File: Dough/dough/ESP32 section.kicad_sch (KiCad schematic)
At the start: 27 parts, among them J12 Conn_01x10_Pin, J401 SD CARD, Q1 2N7002, Q4 2N7002, SW2 ESP32 BOOT, SW4 ESP32 RST, U9 ESP32-S3-WROOM-1

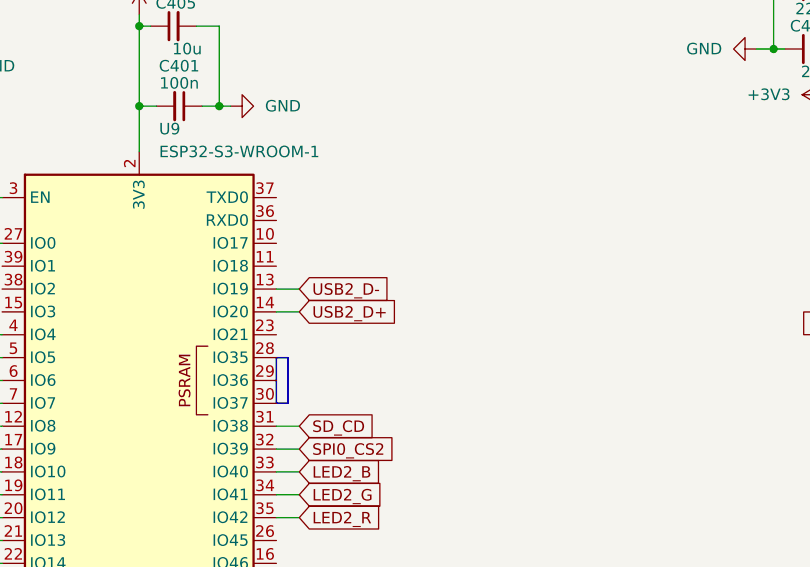
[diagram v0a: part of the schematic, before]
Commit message: started routing
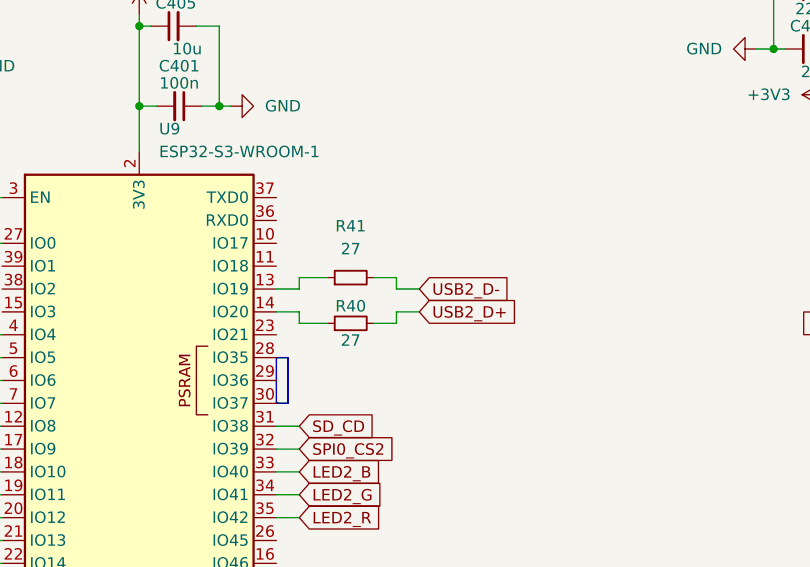
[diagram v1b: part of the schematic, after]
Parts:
- added R40, R41: 27, Resistor_SMD:R_0603_1608Metric_Pad0.98x0.95mm_HandSolder, symbol Device:R_Small
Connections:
- net USB2_D+: now also R40.2; no longer U9.14 (IO20)
- net USB2_D-: now also R41.2; no longer U9.13 (IO19)
- new net: R41.1, U9.13 (IO19)
- new net: R40.1, U9.14 (IO20)
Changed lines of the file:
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@@
+	(wire
+		(pts
+			(xy 154.94 79.375) (xy 151.765 79.375)
+		)
+		(stroke
+			(width 0)
+			(type default)
+		)
+	)
 	(wire
 		(pts
@@
 	(wire
 		(pts
+			(xy 162.56 74.295) (xy 162.56 75.565)
+		)
+		(stroke
+			(width 0)
+			(type default)
+		)
+	)
+	(wire
+		(pts
 			(xy 102.235 66.04) (xy 102.235 73.025)
 		)
@@
 	(wire
 		(pts
+			(xy 149.225 75.565) (xy 151.765 75.565)
+		)
+		(stroke
+			(width 0)
+			(type default)
+		)
+	)
+	(wire
+		(pts
 			(xy 92.075 63.5) (xy 92.075 50.8)
 		)
@@
 	(wire
 		(pts
+			(xy 160.02 79.375) (xy 162.56 79.375)
+		)
+		(stroke
+			(width 0)
+			(type default)
+		)
+	)
+	(wire
+		(pts
 			(xy 204.47 48.895) (xy 205.74 48.895)
 		)
@@
 	(wire
 		(pts
+			(xy 151.765 75.565) (xy 151.765 74.295)
+		)
+		(stroke
+			(width 0)
+			(type default)
+		)
+	)
+	(wire
+		(pts
 			(xy 219.075 84.455) (xy 219.075 81.915)
 		)
@@
 	(wire
 		(pts
+			(xy 151.765 74.295) (xy 154.94 74.295)
+		)
+		(stroke
+			(width 0)
+			(type default)
+		)
+	)
+	(wire
+		(pts
 			(xy 116.84 80.645) (xy 118.745 80.645)
 		)
@@
 	(wire
 		(pts
+			(xy 151.765 78.105) (xy 149.225 78.105)
+		)
+		(stroke
+			(width 0)
+			(type default)
+		)
+	)
+	(wire
+		(pts
 			(xy 204.47 29.845) (xy 204.47 34.925)
 		)
@@
 	(wire
 		(pts
+			(xy 162.56 75.565) (xy 165.1 75.565)
+		)
+		(stroke
+			(width 0)
+			(type default)
+		)
+	)
+	(wire
+		(pts
 			(xy 45.085 21.59) (xy 49.53 21.59)
 		)
@@
 	(wire
 		(pts
+			(xy 151.765 79.375) (xy 151.765 78.105)
+		)
+		(stroke
+			(width 0)
+			(type default)
+		)
+	)
+	(wire
+		(pts
 			(xy 151.765 98.425) (xy 149.225 98.425)
 		)
@@
 	(wire
 		(pts
-			(xy 151.765 78.105) (xy 149.225 78.105)
+			(xy 160.02 74.295) (xy 162.56 74.295)
 		)
 		(stroke
@@
 	(wire
 		(pts
+			(xy 162.56 78.105) (xy 165.1 78.105)
+		)
+		(stroke
+			(width 0)
+			(type default)
+		)
+	)
+	(wire
+		(pts
 			(xy 70.485 55.88) (xy 76.2 55.88)
 		)
@@
 	(wire
 		(pts
-			(xy 151.765 75.565) (xy 149.225 75.565)
+			(xy 162.56 79.375) (xy 162.56 78.105)
 		)
 		(stroke
@@
 	(global_label "USB2_D+"
 		(shape input)
-		(at 151.765 78.105 0)
+		(at 165.1 78.105 0)
 		(fields_autoplaced yes)
 		(effects
@@
 		)
 		(property "Intersheetrefs" "${INTERSHEET_REFS}"
-			(at 163.5797 78.105 0)
+			(at 176.9147 78.105 0)
 			(effects
 				(font
@@
 	(global_label "USB2_D-"
 		(shape input)
-		(at 151.765 75.565 0)
+		(at 165.1 75.565 0)
 		(fields_autoplaced yes)
 		(effects
@@
 		)
 		(property "Intersheetrefs" "${INTERSHEET_REFS}"
-			(at 163.5797 75.565 0)
+			(at 176.9147 75.565 0)
 			(effects
 				(font
@@
 	)
 	(symbol
+		(lib_id "Device:R_Small")
+		(at 157.48 74.295 90)
+		(unit 1)
+		(exclude_from_sim no)
+		(in_bom yes)
+		(on_board yes)
+		(dnp no)
+		(fields_autoplaced yes)
+		(property "Reference" "R41"
+			(at 157.48 68.58 90)
+			(effects
+				(font
+					(size 1.27 1.27)
+				)
+			)
+		)
+		(property "Value" "27"
+			(at 157.48 71.12 90)
+			(effects
+				(font
+					(size 1.27 1.27)
+				)
+			)
+		)
+		(property "Footprint" "Resistor_SMD:R_0603_1608Metric_Pad0.98x0.95mm_HandSolder"
+			(at 157.48 74.295 0)
+			(effects
+				(font
+					(size 1.27 1.27)
+				)
+				(hide yes)
+			)
+		)
+		(property "Datasheet" "~"
+			(at 157.48 74.295 0)
+			(effects
+				(font
+					(size 1.27 1.27)
+				)
+				(hide yes)
+			)
+		)
+		(property "Description" "Resistor, small symbol"
+			(at 157.48 74.295 0)
+			(effects
+				(font
+					(size 1.27 1.27)
+				)
+				(hide yes)
+			)
+		)
+		(pin "2"
+		)
+		(pin "1"
+		)
+		(instances
+			(project "dough"
+				(path "/4fefffc5-b577-4f4a-9ede-53ada2aa57cf/22e4c3eb-dc28-4f86-950b-d0bb031ef536"
+					(reference "R41")
+					(unit 1)
+				)
+			)
+		)
+	)
+	(symbol
 		(lib_id "power:GND")
 		(at 81.28 73.025 270)
@@
 					(unit 1)
 				)
+			)
+		)
+	)
+	(symbol
+		(lib_id "Device:R_Small")
+		(at 157.48 79.375 90)
+		(unit 1)
+		(exclude_from_sim no)
+		(in_bom yes)
+		(on_board yes)
+		(dnp no)
+		(property "Reference" "R40"
+			(at 157.48 77.47 90)
+			(effects
+				(font
+					(size 1.27 1.27)
+				)
+			)
+		)
+		(property "Value" "27"
+			(at 157.48 81.28 90)
+			(effects
+				(font
+					(size 1.27 1.27)
+				)
+			)
+		)
+		(property "Footprint" "Resistor_SMD:R_0603_1608Metric_Pad0.98x0.95mm_HandSolder"
+			(at 157.48 79.375 0)
+			(effects
+				(font
+					(size 1.27 1.27)
+				)
+				(hide yes)
+			)
+		)
+		(property "Datasheet" "~"
+			(at 157.48 79.375 0)
+			(effects
+				(font
+					(size 1.27 1.27)
+				)
+				(hide yes)
+			)
+		)
+		(property "Description" "Resistor, small symbol"
+			(at 157.48 79.375 0)
+			(effects
+				(font
+					(size 1.27 1.27)
+				)
+				(hide yes)
+			)
+		)
+		(pin "2"
+		)
+		(pin "1"
+		)
+		(instances
+			(project "dough"
+				(path "/4fefffc5-b577-4f4a-9ede-53ada2aa57cf/22e4c3eb-dc28-4f86-950b-d0bb031ef536"
+					(reference "R40")
+					(unit 1)
+				)

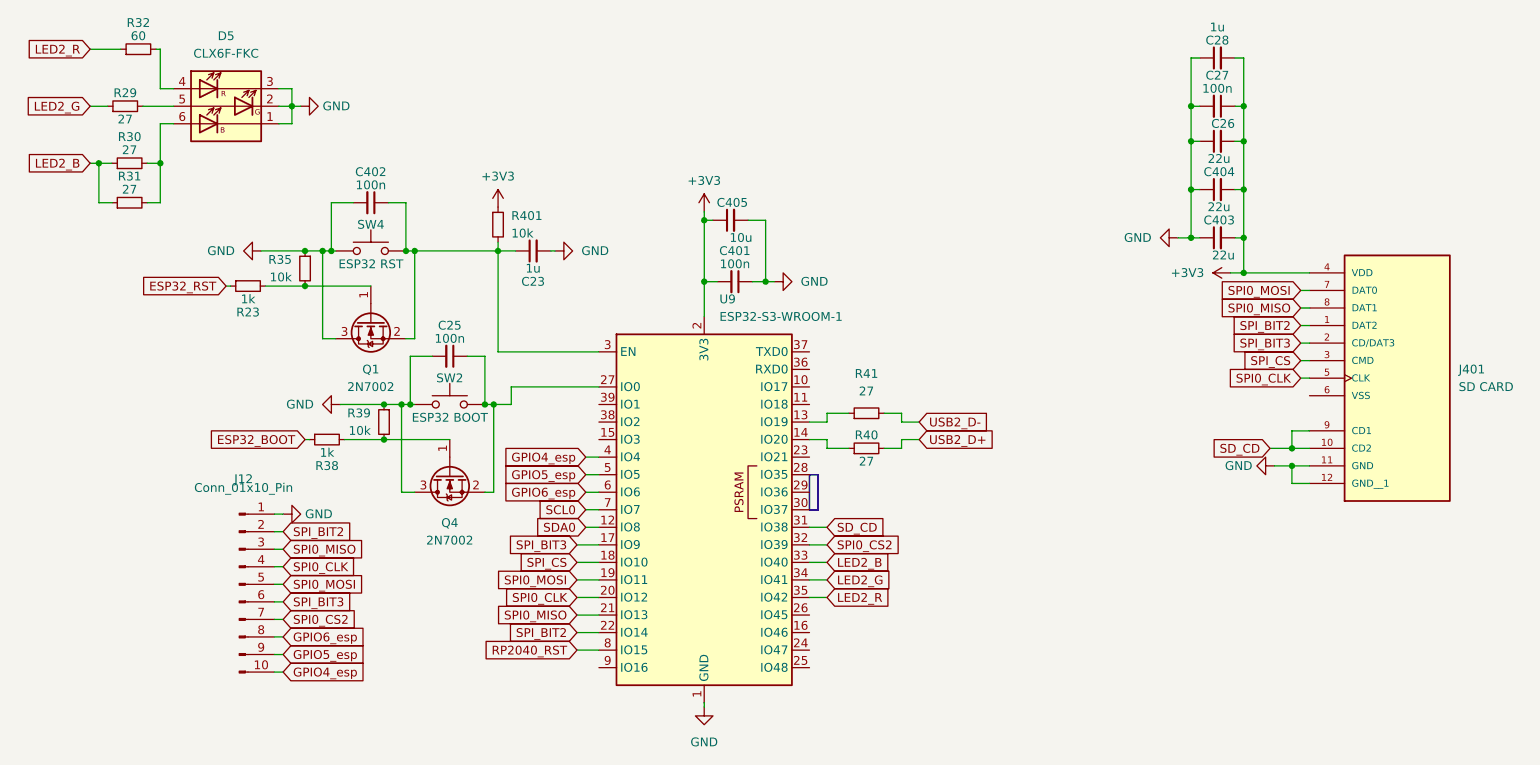
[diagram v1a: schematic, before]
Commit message: pre prod 1
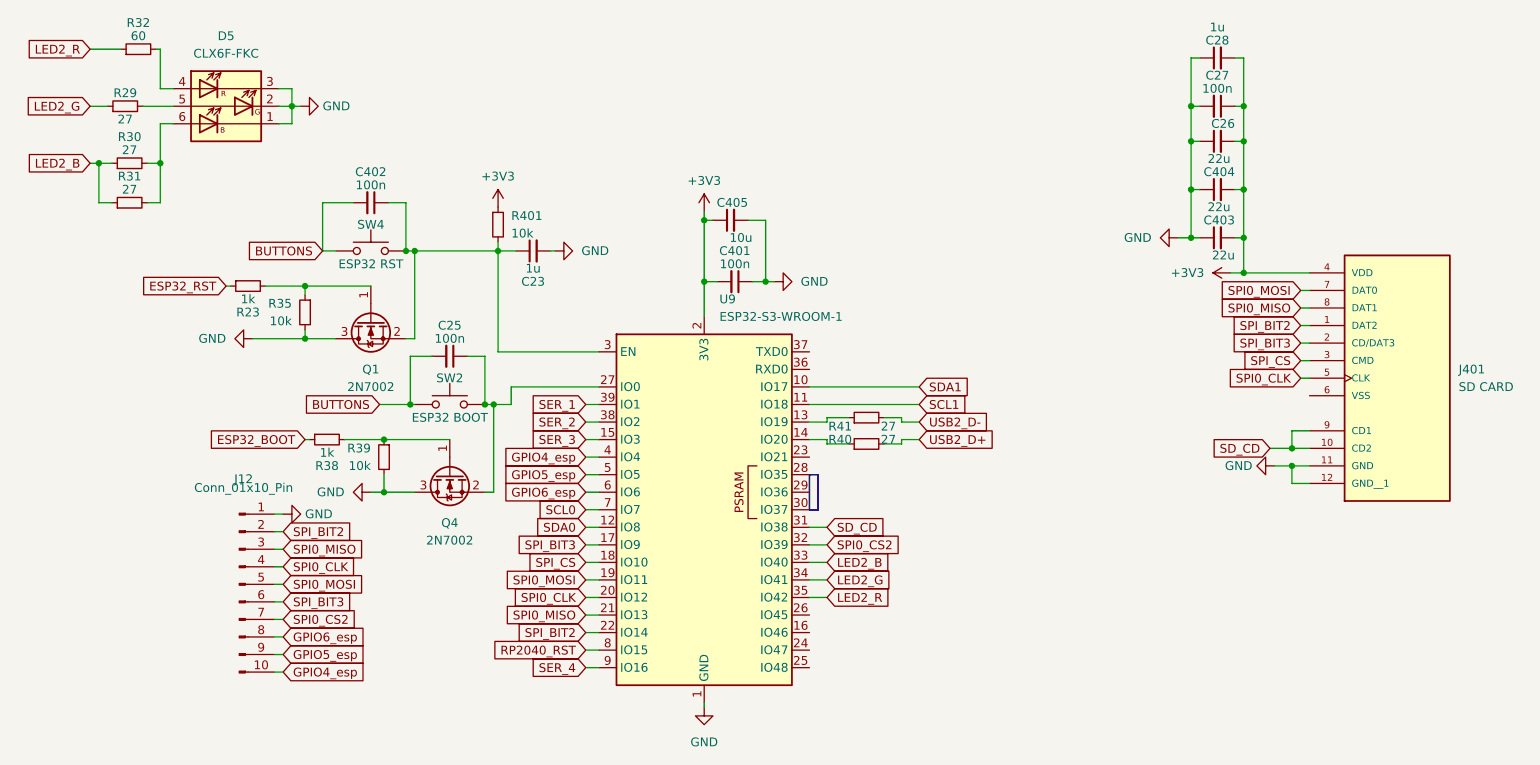
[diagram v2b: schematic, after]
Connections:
- net GND: now also R35.2, R39.2; no longer C25.2, C402.2, R35.1, R39.1, SW2.1, SW4.1
- net at Q1.1 (G), R23.2: now also R35.1; no longer R35.2
- net at Q4.1 (G), R38.2: now also R39.1; no longer R39.2
- net SDA1: now reaches U9.10 (IO17)
- net SCL1: now reaches U9.11 (IO18)
- net SER_3: now reaches U9.15 (IO3)
- net SER_2: now reaches U9.38 (IO2)
- net SER_1: now reaches U9.39 (IO1)
- net SER_4: now reaches U9.9 (IO16)
- new net BUTTONS: C25.2, C402.2, SW2.1, SW4.1
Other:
- moved on the sheet: R40, R41

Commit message: dough First production run
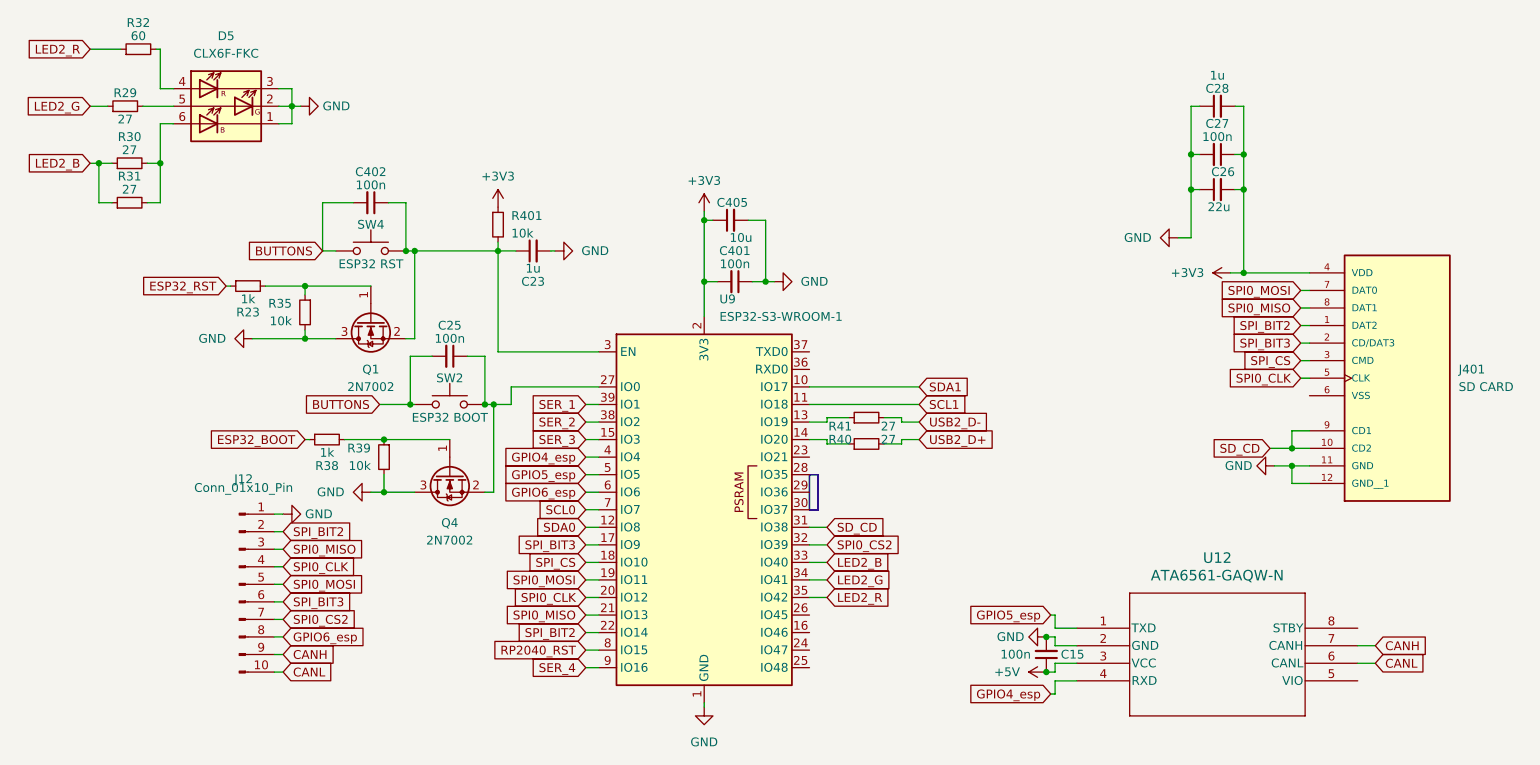
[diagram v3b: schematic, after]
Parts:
- removed C403, C404: 22u, Capacitor_SMD:C_0603_1608Metric_Pad1.08x0.95mm_HandSolder, symbol Device:C_Small
- added C15: 100n, Capacitor_SMD:C_0603_1608Metric_Pad1.08x0.95mm_HandSolder, symbol Device:C_Small
- added U12: ATA6561-GAQW-N, ATA6561_GAQW:SOIC8_4P9X3P9MC_MCH, symbol 2024-08-18_13-36-55:ATA6561-GAQW-N
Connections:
- net GND: now also C15.2, U12.2 (GND)
- net GPIO4_esp: now also U12.4 (RXD); no longer J12.10 (Pin_10)
- net GPIO5_esp: now also U12.1 (TXD); no longer J12.9 (Pin_9)
- new net +5V: C15.1, U12.3 (VCC)
- new net CANH: J12.9 (Pin_9), U12.7 (CANH)
- new net CANL: J12.10 (Pin_10), U12.6 (CANL)
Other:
- moved on the sheet: C26, C27, C28
